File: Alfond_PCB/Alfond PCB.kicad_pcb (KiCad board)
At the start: 2 copper layers, 84.5 x 50 mm, 48 parts, among them J3 Conn_01x05_Pin, J5 USB_B_Micro, P1 PHR-2, SW1 SW_SPDT, U1 DS18B20, U2 STM32U545VETx, U5 MIC5219-3.3YM5-TR, Y1 16MHz

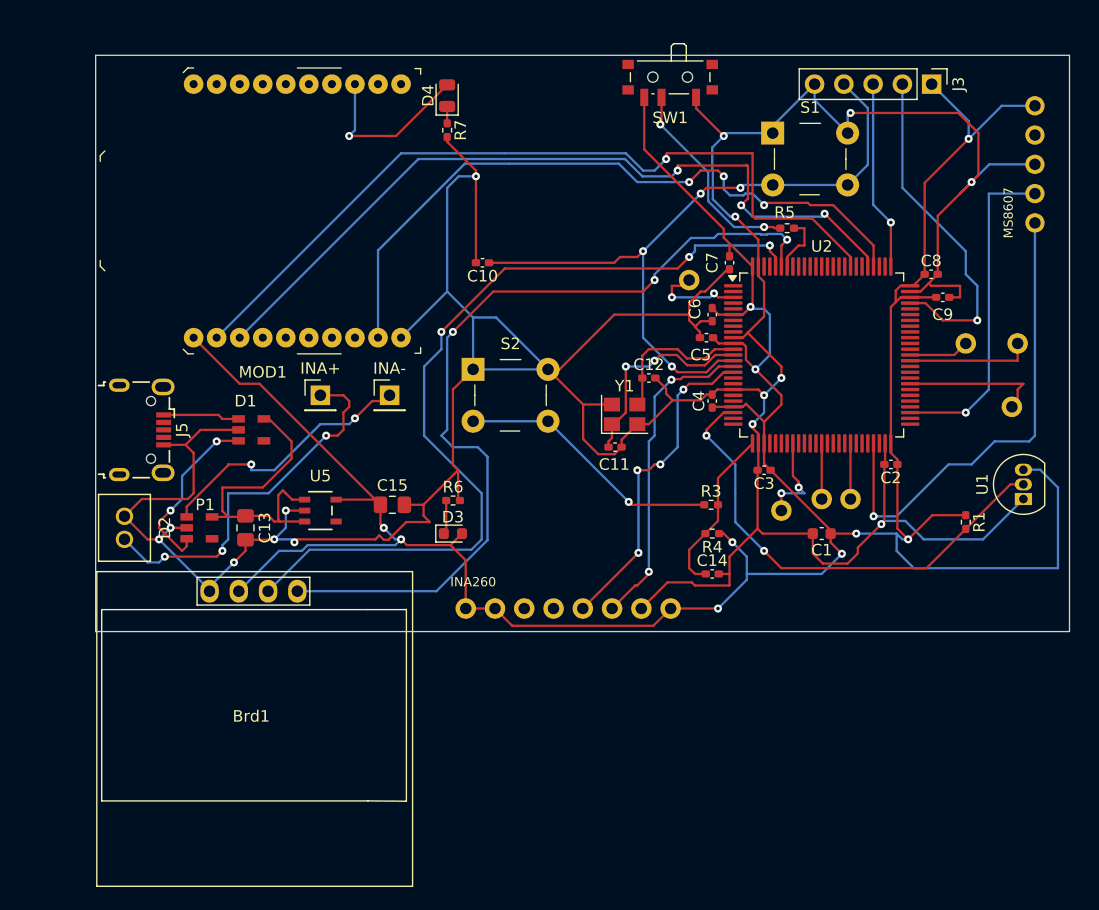
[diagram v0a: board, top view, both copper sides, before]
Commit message: made improvments to pcb
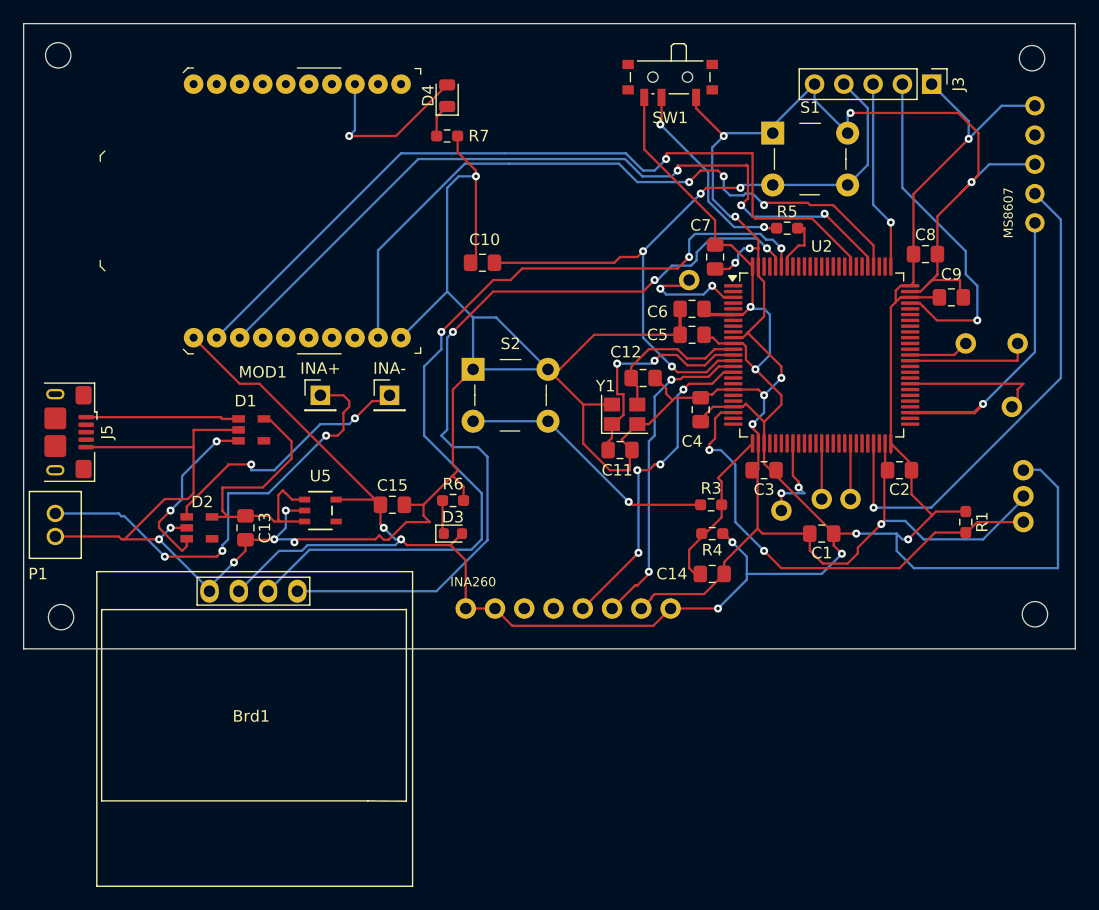
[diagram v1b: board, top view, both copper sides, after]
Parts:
- removed U1: DS18B20, Package_TO_SOT_THT:TO-92_Inline
- added ?: , , F.Cu at (241.5, 86.2)
- added ?: , , F.Cu at (241.5, 84.0)
- added ?: , , F.Cu at (241.5, 88.5)
- added H1: MountingHole, MountingHole:MountingHole_2.2mm_M2, F.Cu at (157.8, 48.0)
- added H2: MountingHole, MountingHole:MountingHole_2.2mm_M2, F.Cu at (242.2, 48.2)
- added H3: MountingHole, MountingHole:MountingHole_2.2mm_M2, F.Cu at (158.0, 96.8)
- added H4: MountingHole, MountingHole:MountingHole_2.2mm_M2, F.Cu at (242.5, 96.5)
- C1: footprint Capacitor_SMD:C_0603_1608Metric -> Capacitor_SMD:C_0805_2012Metric_Pad1.18x1.45mm_HandSolder
- C10, C11, C12, C14, C2, C3, C4, C5, C6, C7, C8, C9: footprint Capacitor_SMD:C_0402_1005Metric_Pad0.74x0.62mm_HandSolder -> Capacitor_SMD:C_0805_2012Metric_Pad1.18x1.45mm_HandSolder
- J5: footprint Connector_USB:USB_Micro-B_Wuerth_629105150521 -> Connector_USB:USB_Micro-B_Amphenol_10118193-0001LF_Horizontal
- R1, R3, R4, R5, R6, R7: footprint Resistor_SMD:R_0402_1005Metric_Pad0.72x0.64mm_HandSolder -> Resistor_SMD:R_0603_1608Metric_Pad0.98x0.95mm_HandSolder
- moved J5 7.50 mm to (157.5, 80.7)
- moved P1 6.01 mm to (157.5, 88.8), turned to 90 degrees
- moved C6 1.82 mm to (212.8, 70.0), turned to 180 degrees
- moved C8 1.82 mm to (233.0, 65.2)
- moved C7 1.35 mm to (214.8, 65.5)
- moved C5 1.27 mm to (212.8, 72.2)
- moved C4 1.25 mm to (213.5, 78.8)
- moved C2 0.90 mm to (230.8, 84.0)
- moved C9 0.75 mm to (235.2, 69.0)
- moved C12 0.50 mm to (208.5, 76.0)
- moved R7 0.50 mm to (191.5, 55.0), turned to 0 degrees
- moved C11 0.50 mm to (206.5, 82.2)
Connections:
- U2 pad 47: /I2C2_SDA -> /I2C2_SCL
- U2 pad 53: /I2C2_SCL -> /I2C2_SDA
- U2 pad 95: /I2C1_SDA -> /I2C1_SCL
- U2 pad 96: /I2C1_SCL -> /I2C1_SDA
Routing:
- net /I2C2_SDA: track 41.7 -> 24.2 mm
- net /I2C2_SCL: track 28.7 -> 43.4 mm
- net GND: track 342.0 -> 354.6 mm, vias 15 -> 17
- net /V_USB: track 6.64 -> 13.3 mm
- net /INA+: track 32.6 -> 39.2 mm
- net +3.3V: track 259.5 -> 262.5 mm
- net /I2C1_SDA: track 75.3 -> 73.0 mm
- net /I2C1_SCL: track 75.0 -> 77.1 mm
- net unconnected-(U2-PE4-Pad3): track 8.32 -> 10.1 mm
- net /HSE_OUT: track 18.2 -> 19.8 mm
- net /PWR_LED_K2: track 1.47 -> 2.94 mm
- net /HSE_IN: track 13.2 -> 14.3 mm
- net /UART4_TX: track 41.7 -> 40.8 mm
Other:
- board size 84.5 x 50 mm -> 91.2 x 54.2 mm
